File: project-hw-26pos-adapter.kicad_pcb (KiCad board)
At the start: 4 copper layers, 38 x 52 mm, 4 parts, among them J1 SM04B-SRSS-TB(LF)(SN), J2 3220-26-0300-00, U1 Pink Panda v2.1.0

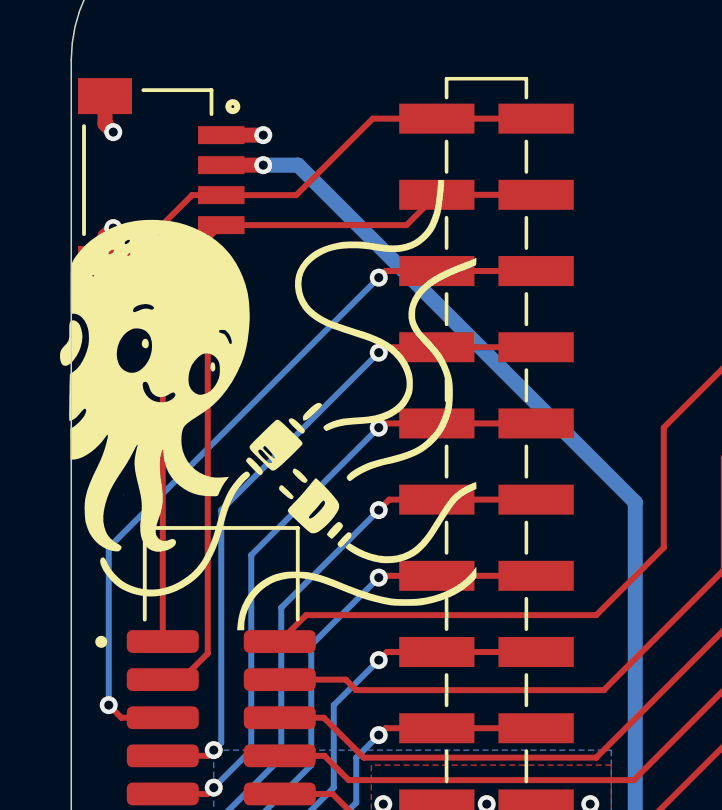
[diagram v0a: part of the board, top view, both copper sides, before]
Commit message: Print 1:1
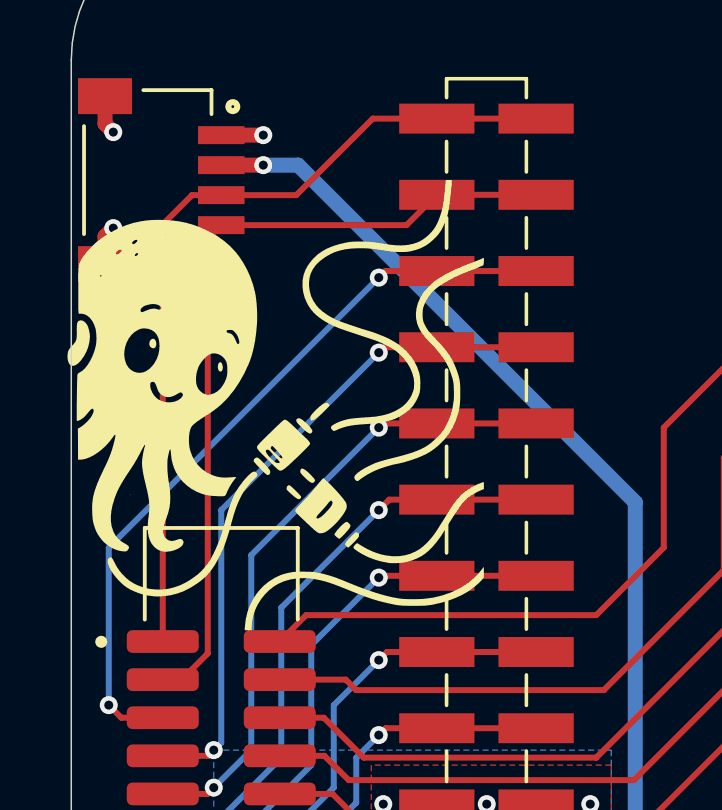
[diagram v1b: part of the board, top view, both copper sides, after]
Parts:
- moved G*** 0.25 mm to (38.2, 35.5)
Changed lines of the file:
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@@
 	(footprint "logos:octopus_15mm"
 		(layer "F.Cu")
-		(at 38 35.5)
+		(at 38.25 35.5)
 		(property "Reference" "G***"
 			(at 0 0 0)
